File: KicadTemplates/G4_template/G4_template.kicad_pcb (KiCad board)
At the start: 2 copper layers, 71.1 x 83.2 mm, 10 parts, among them J1 Conn_01x04_Female, J2 Conn_01x03_Male, J3 Conn_01x03_Male, J4 Conn_02x10_Odd_Even, J5 Conn_02x03_Odd_Even, J6 Conn_01x01_Female, SW1 SW_SPDT, U2 NUCLEO-G491RE

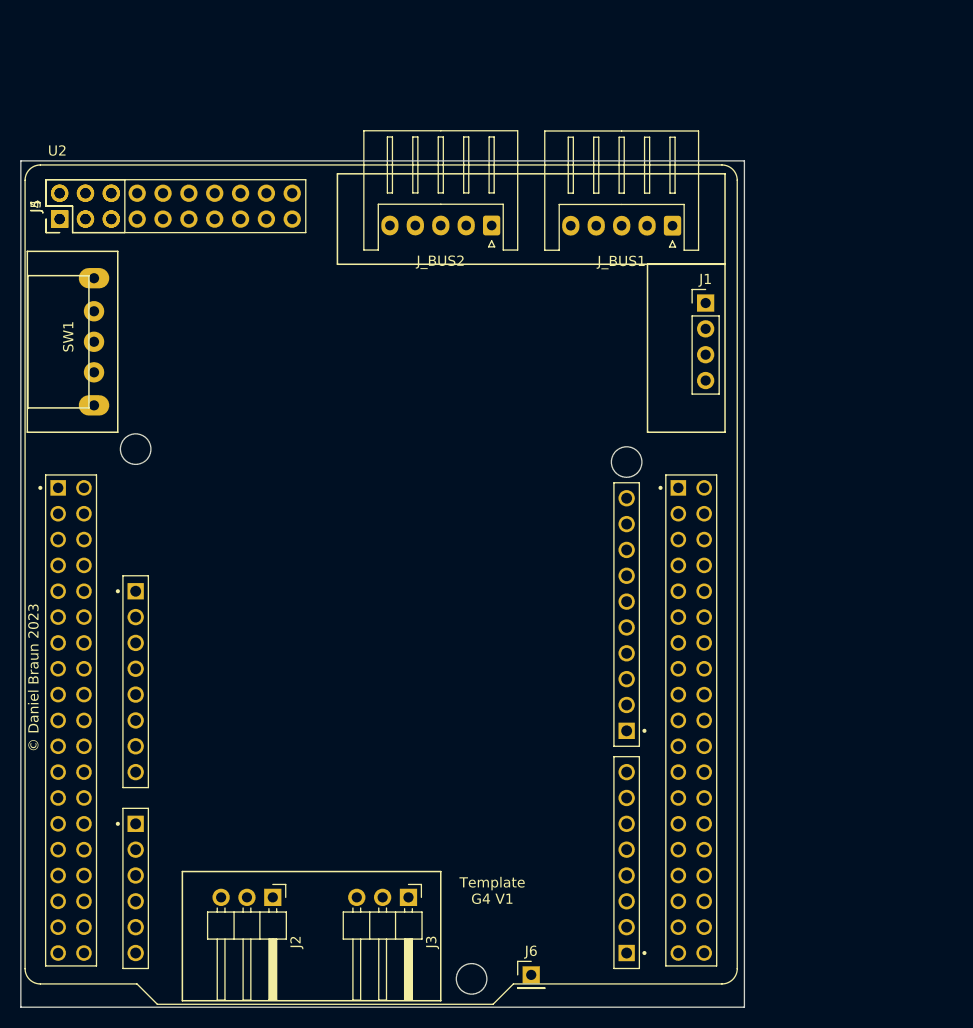
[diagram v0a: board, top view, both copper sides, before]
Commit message: updated template
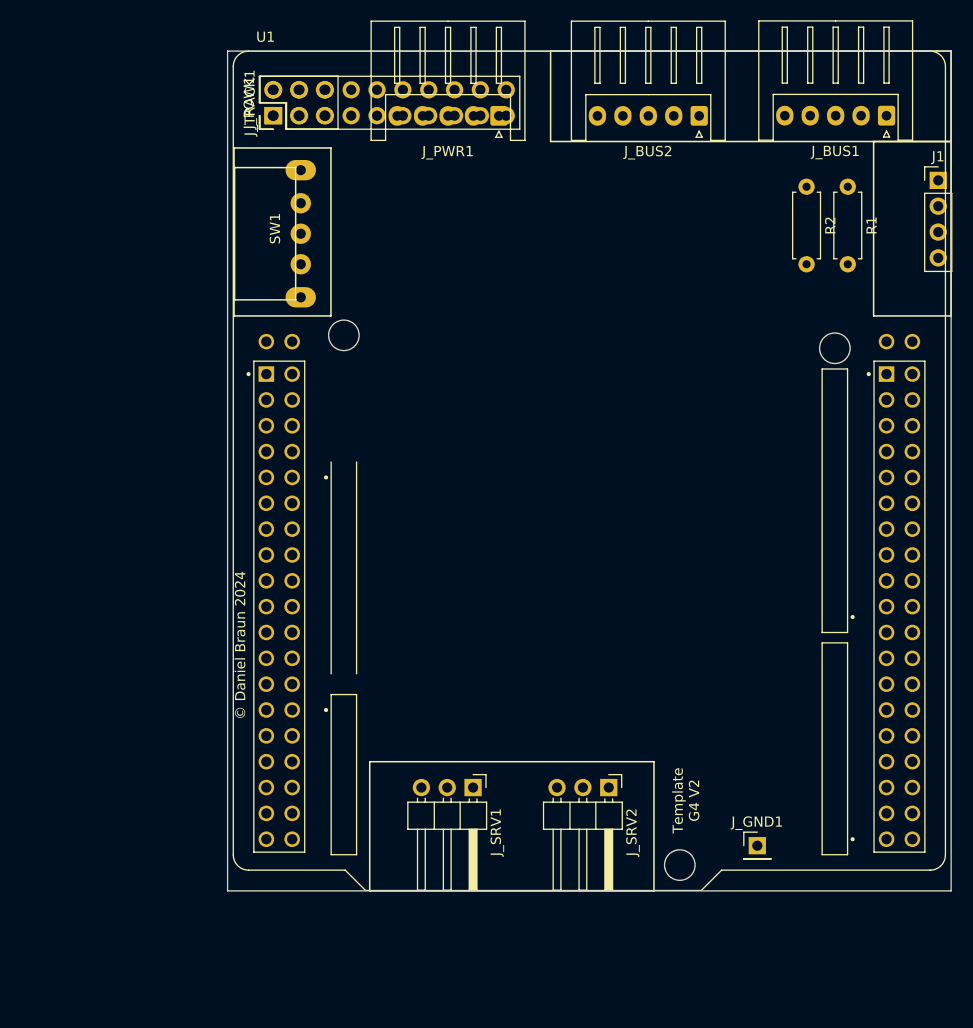
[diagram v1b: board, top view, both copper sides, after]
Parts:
- removed U2: NUCLEO-G491RE, G4Lib:MODULE_NUCLEO-G491RE
- added J_PWR1: Conn_01x05_Female, Connector_JST:JST_XH_S5B-XH-A_1x05_P2.50mm_Horizontal, F.Cu at (118.7, 59.1)
- added R1: 4.4K, Resistor_THT:R_Axial_DIN0207_L6.3mm_D2.5mm_P7.62mm_Horizontal, F.Cu at (153.0, 66.0)
- added R2: 4.4K, Resistor_THT:R_Axial_DIN0207_L6.3mm_D2.5mm_P7.62mm_Horizontal, F.Cu at (149.0, 66.0)
- added U1: NUCLEO-G491RE, G4Lib:MODULE_NUCLEO-G491RE20, F.Cu at (127.6, 94.0)
- moved J1 25.8 mm to (161.9, 65.4)
- moved J_GND1 25.6 mm to (144.1, 130.8)
- moved J_BUS1 23.7 mm to (156.8, 59.1)
- moved J_TRACK1 23.4 mm to (96.6, 59.1)
- moved J_POW1 23.3 mm to (96.5, 59.1)
- moved J_BUS2 23.1 mm to (138.4, 59.1)
- moved SW1 22.9 mm to (99.3, 70.7)
- moved J_SRV1 22.5 mm to (116.2, 125.1)
- moved J_SRV2 22.5 mm to (129.5, 125.1)
- renumbered J6 to J_GND1, J5 to J_POW1, J2 to J_SRV1, J3 to J_SRV2, J4 to J_TRACK1
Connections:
- net Net-(J_BUS1-Pad4) renamed CANH
- net Net-(J_BUS1-Pad5) renamed CANL
- J1 pad 1: unconnected-(J1-Pad1) -> I2C3_DTA
- J1 pad 2: unconnected-(J1-Pad2) -> I2C3_CK
- J1 pad 3: unconnected-(J1-Pad3) -> 3V3
- J1 pad 4: unconnected-(J1-Pad4) -> GND
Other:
- board size 71.1 x 83.2 mm -> 71.1 x 82.5 mm
- board text added: "Template G4 V2"
- board text added: "© Daniel Braun 2024"
- board text removed: "Template G4 V1"
- board text removed: "© Daniel Braun 2023"
